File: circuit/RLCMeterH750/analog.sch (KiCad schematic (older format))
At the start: 33 parts

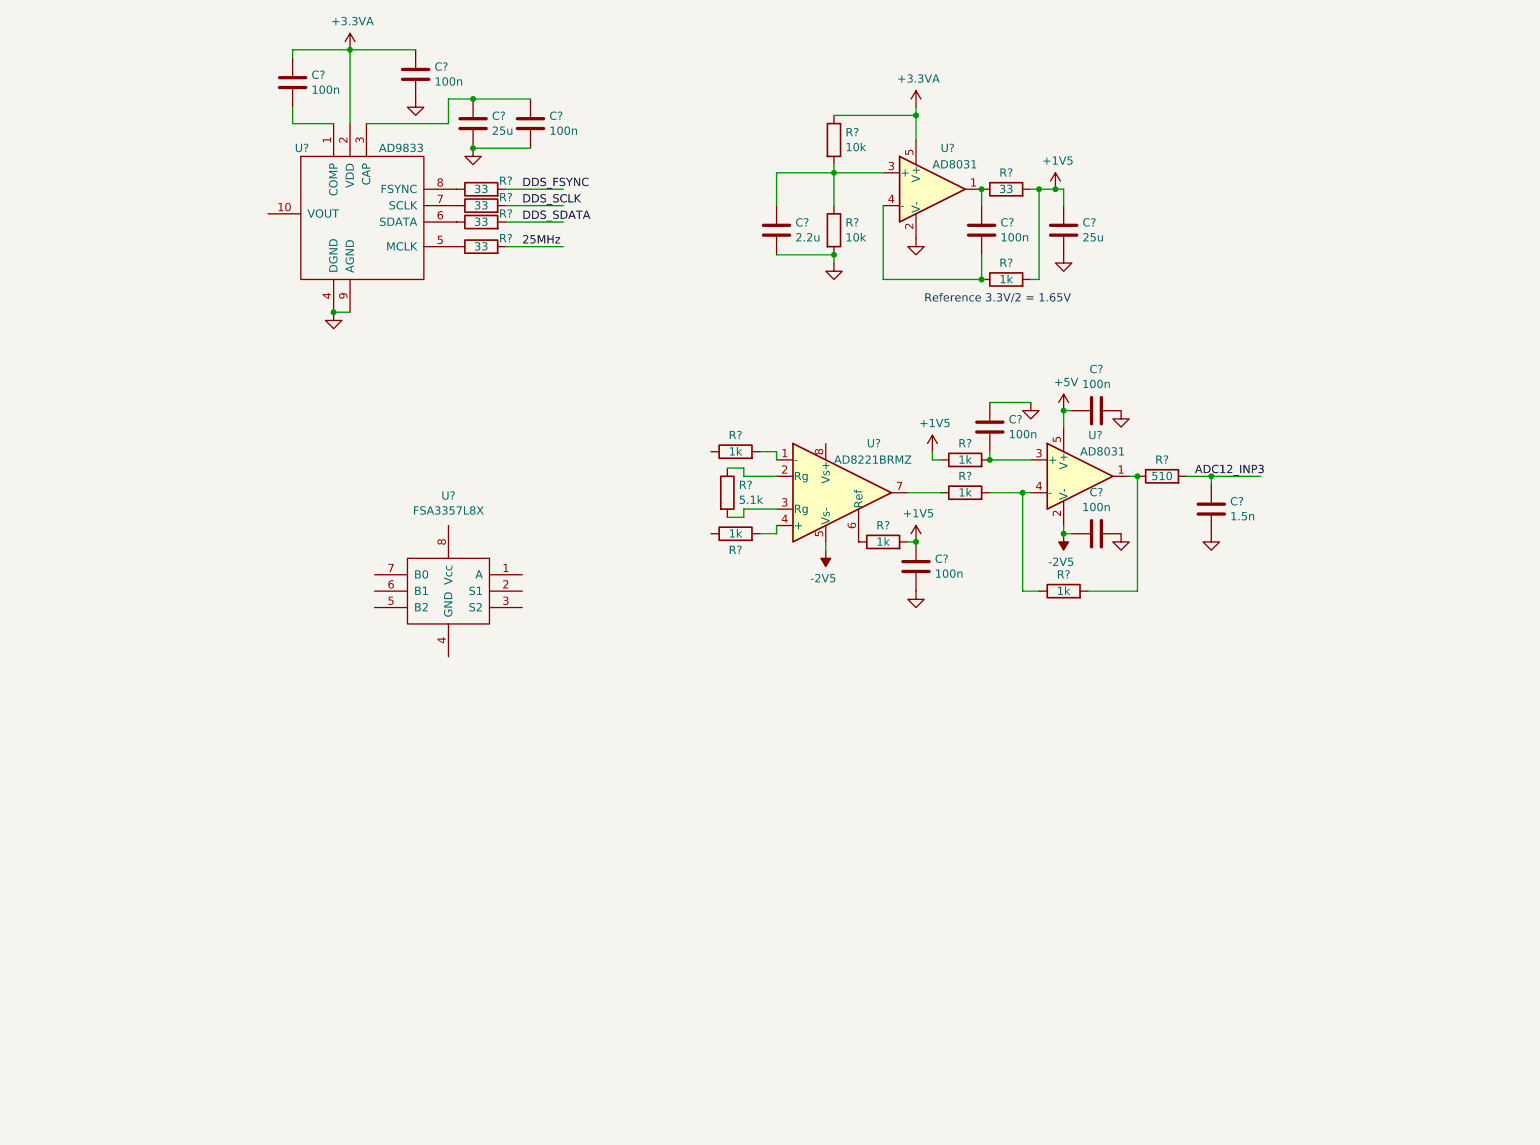
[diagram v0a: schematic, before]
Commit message: - вродебы нарисовали аналоговую часть
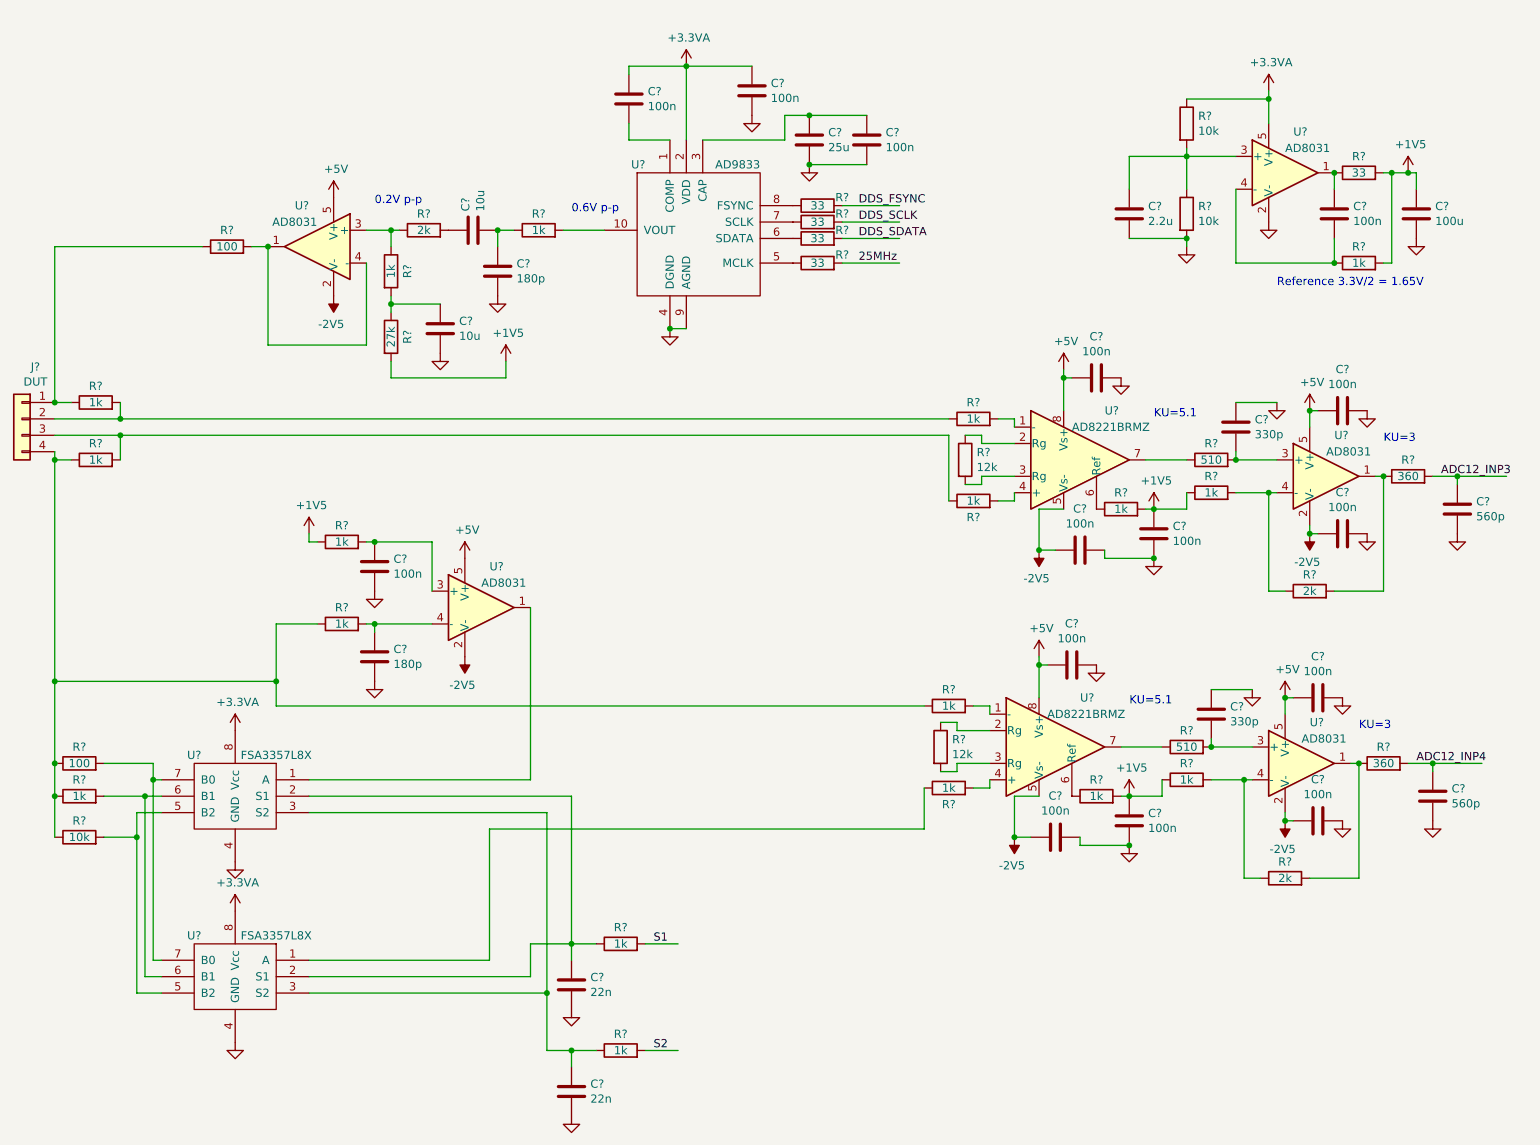
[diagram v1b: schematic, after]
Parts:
- removed C?: 100n, symbol Device:C
- added C? (x8): 100n, Capacitor_SMD:C_0603_1608Metric, symbol Device:C
- added C? (x2): 330p, Capacitor_SMD:C_1206_3216Metric, symbol Device:C
- added C? (x2): 22n, Capacitor_SMD:C_0603_1608Metric, symbol Device:C
- added C?: 560p, Capacitor_SMD:C_1206_3216Metric, symbol Device:C
- added C? (x2): 180p, Capacitor_SMD:C_1206_3216Metric, symbol Device:C
- added C? (x2): 10u, Capacitor_SMD:C_1206_3216Metric, symbol Device:C
- added J?: DUT, Connector_PinHeader_2.54mm:PinHeader_1x04_P2.54mm_Vertical, symbol Connector_Generic:Conn_01x04
- added R? (x13): 1k, Resistor_SMD:R_0603_1608Metric, symbol Device:R
- added R? (x2): 2k, Resistor_SMD:R_0603_1608Metric, symbol Device:R
- added R?: 360, Resistor_SMD:R_0603_1608Metric, symbol Device:R
- added R?: 510, Resistor_SMD:R_0603_1608Metric, symbol Device:R
- added R?: 12k, Resistor_SMD:R_0603_1608Metric, symbol Device:R
- added R? (x2): 100, Resistor_SMD:R_0603_1608Metric, symbol Device:R
- added R?: 27k, Resistor_SMD:R_0603_1608Metric, symbol Device:R
- added R?: 10k, Resistor_SMD:R_0603_1608Metric, symbol Device:R
- added U? (x3): AD8031, Package_TO_SOT_SMD:SOT-23-5, symbol Amplifier_Operational:MCP6001-OT
- added U?: AD8221BRMZ, Package_SO:MSOP-8_3x3mm_P0.65mm, symbol Amplifier_Instrumentation:AD8421BRMZ
- added U?: FSA3357L8X, balmer:MicroPak_8-Lead, symbol balmer:FSA3357L8X
- C?: value 1.5n -> 560p
- C?: value 25u -> 100u
- R?: value 1k -> 2k
- R?: value 510 -> 360
- R?: value 1k -> 510
- R?: value 5.1k -> 12k
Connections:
- net labels added: ADC12_INP4, S1, S2
- wire segments 68 -> 195
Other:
- note added: "0.2V p-p"
- note added: "0.6V p-p"
- note added: "KU=3"
- note added: "KU=5.1"
- moved on the sheet: C?, R?, U?
